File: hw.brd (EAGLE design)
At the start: 80 x 80 mm, 37 parts, among them IC1 MIC_I2S_SPH0645, Q3 DMG3415U, U1 MAX98357A, U2 AP2112-3.3, U3 MCP73831T-2ACI/OT, X2 JSTPH

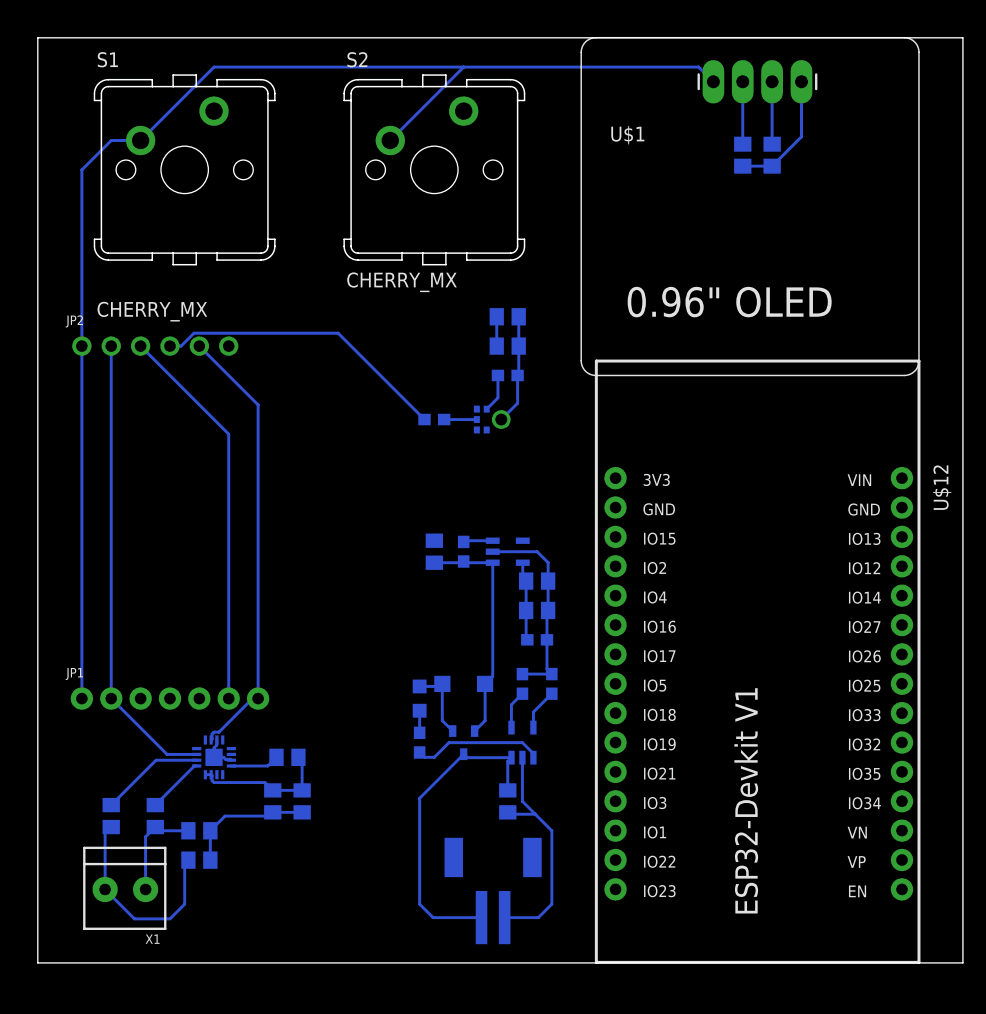
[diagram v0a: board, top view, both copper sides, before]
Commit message: rerouting :|
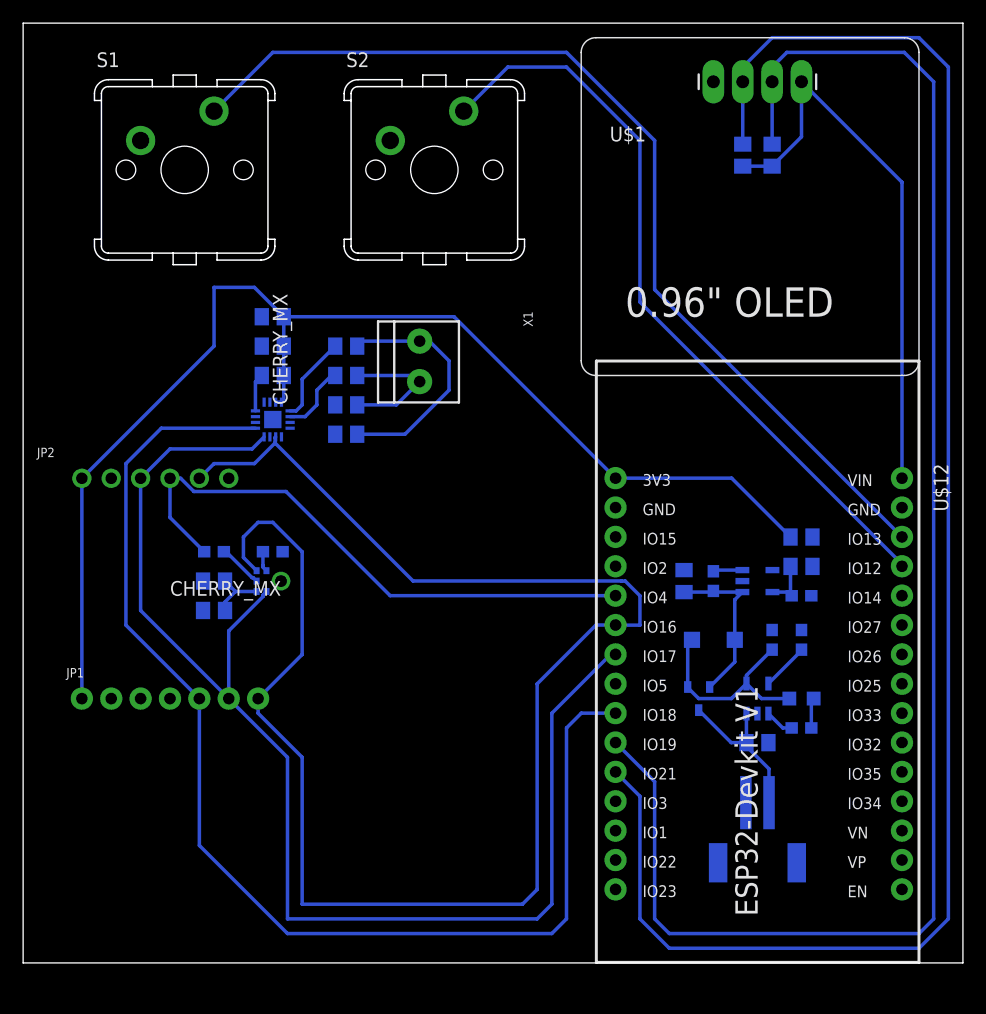
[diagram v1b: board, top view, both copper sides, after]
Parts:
- moved X1 52.3 mm to (33.0, 52.1), turned to 270 degrees
- moved FB1 43.9 mm to (26.7, 53.3), turned to 180 degrees
- moved FB2 43.2 mm to (26.7, 50.8), turned to 180 degrees
- moved C2 41.9 mm to (20.3, 55.9), turned to 0 degrees
- moved C4 41.4 mm to (26.7, 48.3), turned to 0 degrees
- moved C1 39.5 mm to (20.3, 53.3), turned to 0 degrees
- moved C5 36.6 mm to (26.7, 45.7), turned to 0 degrees
- moved C3 34.2 mm to (15.2, 33.0), turned to 0 degrees
- moved C6 34.2 mm to (15.2, 30.5), turned to 0 degrees
- moved R4 33.0 mm to (66.0, 20.3), turned to 0 degrees
- moved R1 33.0 mm to (20.3, 50.8)
- moved CHG 33.0 mm to (66.0, 22.9), turned to 90 degrees
- moved U1 29.6 mm to (20.3, 47.0), turned to 180 degrees
- moved R3 25.4 mm to (20.3, 35.6)
- moved IC1 23.6 mm to (20.3, 33.0)
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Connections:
- removed net N$12: U$12.24
- removed net VCC: R11.2, R9.2, U$1.4
- removed net WS: IC1.1
- net 3.3V: now also C1.1, C2.1, C3.1, C6.1, IC1.5, JP1.1, JP2.1, R1.2, U$12.1, U1.7, U1.8
- net BCLK: now also U$12.7; no longer U$12.21
- net BTN1: now also U$12.27; no longer U$12.15
- net BTN2: now also U$12.28; no longer U$12.14
- net DIN: now also U$12.9; no longer U$12.23
- net DOUT: now also U$12.5; no longer U$12.24
- net GAIN: no longer JP1.4
- net GND: now also U$12.2
- net LRCLK: now also IC1.1, U$12.6; no longer U$12.22
- net SCL: now also U$12.11; no longer U$12.10
- net SDA: now also U$12.10; no longer U$12.11
- net SD_MODE: no longer JP1.3
- net SELECT: no longer JP2.6, U$12.26
- net VDD: now also R11.2, R9.2, U$1.4, U$12.30; no longer C1.1, C2.1, C3.1, C6.1, IC1.5, JP1.1, JP2.1, R1.2, U1.7, U1.8
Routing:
- net GND: track 215.8 -> 0.00 mm
- net SCL: track 5.40 -> 142.6 mm
- net SDA: track 5.40 -> 136.4 mm
- net 3.3V: track 6.83 -> 116.5 mm
- net DIN: track 0.00 -> 104.8 mm
- net LRCLK: track 38.4 -> 141.7 mm
- net BTN2: track 0.00 -> 86.5 mm
- net BCLK: track 33.6 -> 113.6 mm
- net BTN1: track 0.00 -> 65.7 mm
- net VDD: track 14.7 -> 48.8 mm
- net DOUT: track 25.6 -> 50.3 mm
- net VBAT: track 27.6 -> 14.3 mm
- net VO+: track 8.74 -> 20.9 mm
- net VCC: track 10.9 -> 0.00 mm
- net N$3: track 11.3 -> 2.52 mm
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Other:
- board size 80 x 80 mm -> 81.3 x 81.3 mm
